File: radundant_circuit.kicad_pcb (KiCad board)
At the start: 2 copper layers, 57 x 34 mm, 20 parts, among them J1 IN1, J2 IN2, J3 OUT

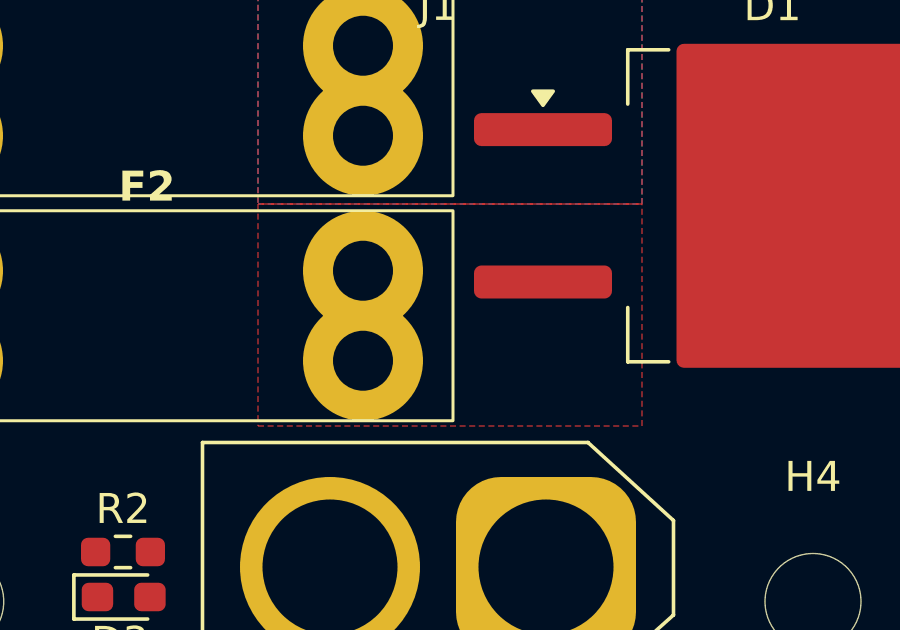
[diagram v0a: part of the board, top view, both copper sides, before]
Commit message: Autosave
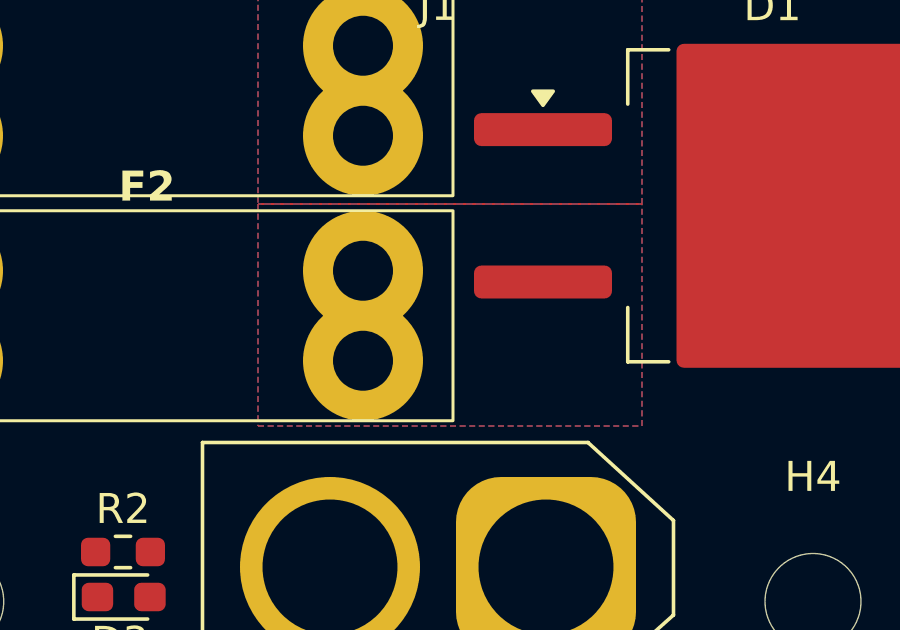
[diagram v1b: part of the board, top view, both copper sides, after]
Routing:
- added copper zone on B.Cu, net IN2
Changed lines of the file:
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@@
+	)
+	(zone
+		(net "IN1")
+		(layers "F.Cu" "B.Cu")
+		(hatch edge 0.5)
+		(connect_pads
+			(clearance 0.5)
+		)
+		(min_thickness 0.25)
+		(fill yes
+			(thermal_gap 0.5)
+			(thermal_bridge_width 0.5)
+			(island_removal_mode 0)
+		)
+		(polygon
+			(pts
+				(xy 53 35.8) (xy 53 43.4) (xy 65.8 43.4) (xy 65.8 35.8)
+			)
+		)
 	)
 	(zone
 		(net "IN2")
-		(layer "F.Cu")
+		(layers "F.Cu" "B.Cu")
 		(hatch edge 0.5)
 		(priority 1)
@@
 		)
 		(min_thickness 0.25)
-		(fill
+		(fill yes
 			(thermal_gap 0.5)
 			(thermal_bridge_width 0.5)
@@
 			)
 		)
-	)
-	(zone
-		(net "IN1")
-		(layers "F.Cu" "B.Cu")
-		(hatch edge 0.5)
-		(connect_pads
-			(clearance 0.5)
-		)
-		(min_thickness 0.25)
-		(fill
-			(thermal_gap 0.5)
-			(thermal_bridge_width 0.5)
-			(island_removal_mode 0)
-		)
-		(polygon
-			(pts
-				(xy 53 35.8) (xy 53 43.4) (xy 65.8 43.4) (xy 65.8 35.8)
-			)
-		)
